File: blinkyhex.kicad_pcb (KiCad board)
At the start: 2 copper layers, 90.5 x 37.9 mm, 124 parts, among them IC1 WS2812B, IC2 ATTINY85-S, K1 D0, K2 A3, K3 A1, K4 A2, K5 reset+in, K6 D1, K7 reset, P1 act-a2, P2 act-a3, P3 act-a1, P4 act-1, P5 act-0, P6 MISO, P7 SCK, P8 MOSI, P9 ISCP

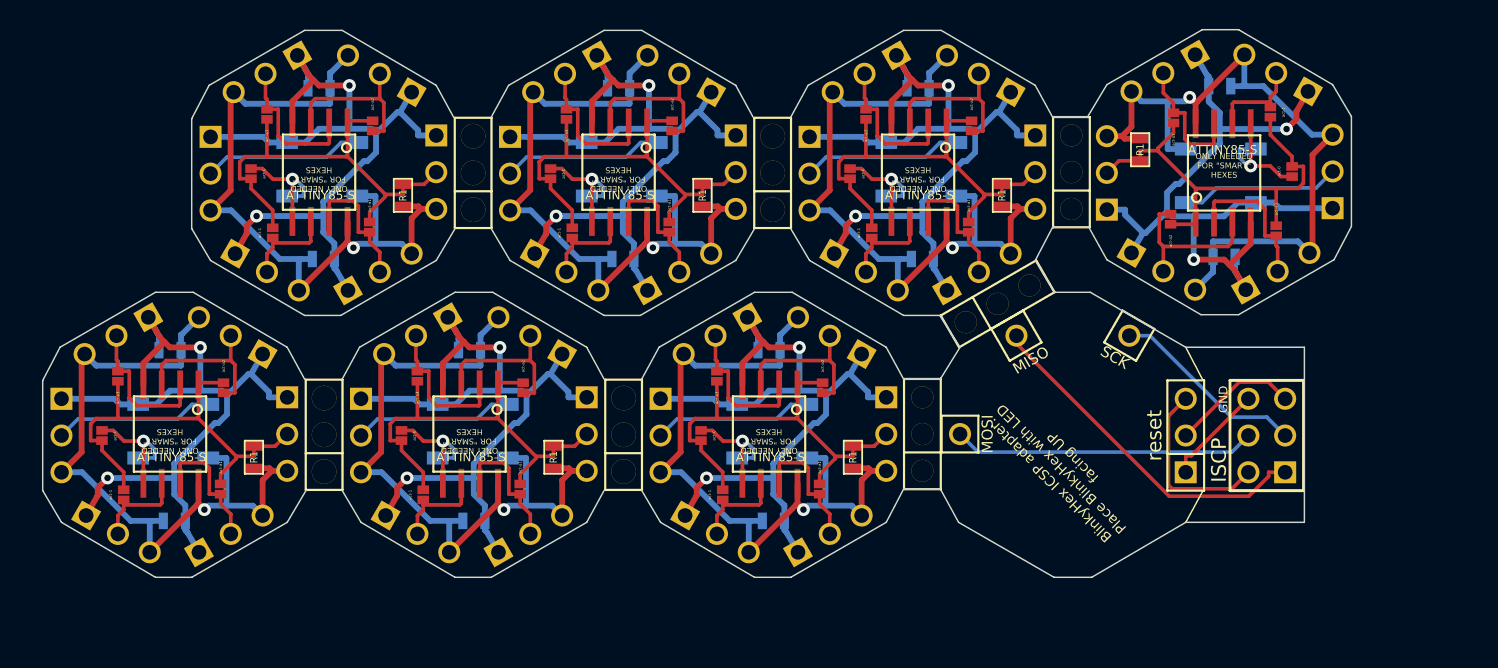
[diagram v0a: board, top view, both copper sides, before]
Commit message: Published.
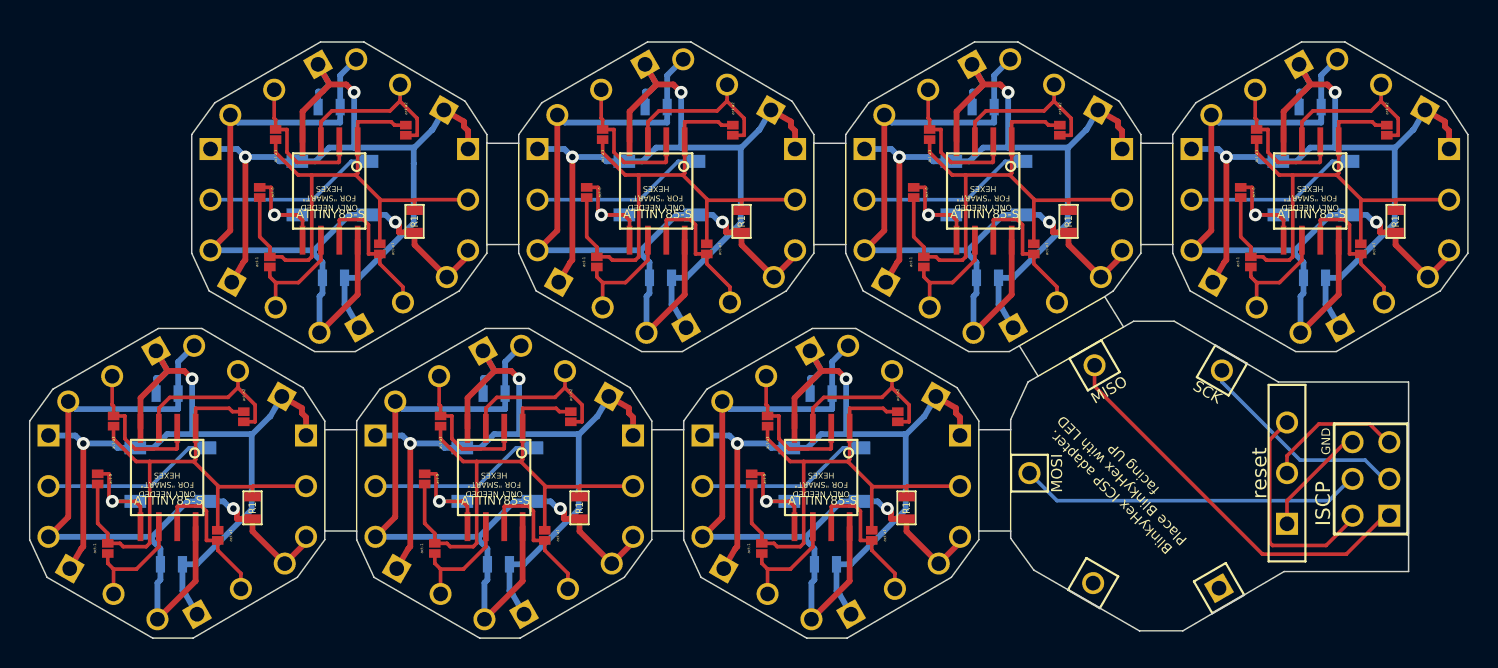
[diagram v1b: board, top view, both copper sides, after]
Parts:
- removed 2, 3, 4, PIN_ARRAY_3X1 (x4): Val**, PIN_ARRAY_3X1
- removed the C1 at (94.8, 28.6)
- removed the C1 at (22.0, 35.0)
- removed the C1 at (42.7, 35.0)
- removed the C1 at (63.4, 35.0)
- removed the C1 at (73.7, 16.9)
- removed the C1 at (53.0, 16.9)
- removed the C2 at (94.5, 16.8)
- removed the C2 at (22.3, 46.8)
- removed the C2 at (43.0, 46.8)
- removed the C2 at (63.7, 46.8)
- removed the C2 at (74.0, 28.7)
- removed the C2 at (53.3, 28.7)
- removed the IC1 at (94.7, 22.9)
- removed the IC1 at (22.2, 40.6)
- removed the IC1 at (42.9, 40.6)
- removed the IC1 at (63.6, 40.6)
- removed the IC1 at (73.9, 22.5)
- removed the IC1 at (53.2, 22.5)
- removed the IC2 at (94.8, 22.6)
- removed the IC2 at (22.1, 40.9)
- removed the IC2 at (42.8, 40.9)
- removed the IC2 at (63.5, 40.9)
- removed the IC2 at (73.8, 22.8)
- removed the IC2 at (53.1, 22.8)
- removed the K1 at (102.3, 22.6)
- removed the K1 at (14.5, 40.9)
- removed the K1 at (35.2, 40.9)
- removed the K1 at (55.9, 40.9)
- removed the K1 at (66.2, 22.8)
- removed the K1 at (45.5, 22.8)
- removed the K1 at (24.8, 22.8)
- removed the K2 at (98.5, 29.6)
- removed the K2 at (18.3, 34.0)
- removed the K2 at (39.0, 34.0)
- removed the K2 at (59.7, 34.0)
- removed the K2 at (70.0, 15.9)
- removed the K2 at (49.3, 15.9)
- removed the K2 at (28.6, 15.9)
- removed the K3 at (90.7, 15.8)
- removed the K3 at (26.2, 47.7)
- removed the K3 at (46.9, 47.7)
- removed the K3 at (67.6, 47.7)
- removed the K3 at (77.9, 29.6)
- removed the K3 at (57.2, 29.6)
- removed the K3 at (36.5, 29.6)
- removed the K4 at (90.7, 29.6)
- removed the K4 at (26.2, 34.0)
- removed the K4 at (46.9, 34.0)
- removed the K4 at (67.6, 34.0)
- removed the K4 at (77.9, 15.9)
- removed the K4 at (57.2, 15.9)
- removed the K4 at (36.5, 15.9)
- removed the K5 at (86.8, 22.8)
- removed the K5 at (30.1, 40.8)
- removed the K5 at (50.8, 40.8)
- removed the K5 at (71.5, 40.8)
- removed the K5 at (81.8, 22.7)
- removed the K5 at (61.1, 22.7)
- removed the K5 at (40.4, 22.7)
- removed the K6 at (98.5, 15.8)
- removed the K6 at (18.4, 47.7)
- removed the K6 at (39.1, 47.7)
- removed the K6 at (59.8, 47.7)
- removed the K6 at (70.1, 29.6)
- removed the K6 at (49.4, 29.6)
- removed the K6 at (28.7, 29.6)
- removed the P1 at (91.2, 25.9)
- removed the P1 at (25.7, 37.6)
- removed the P1 at (46.4, 37.6)
- removed the P1 at (67.1, 37.6)
- removed the P1 at (77.4, 19.5)
- removed the P1 at (56.7, 19.5)
- removed the P2 at (98.5, 26.8)
- removed the P2 at (18.4, 36.8)
- removed the P2 at (39.1, 36.8)
- removed the P2 at (59.8, 36.8)
- removed the P2 at (70.1, 18.7)
- removed the P2 at (49.4, 18.7)
- removed the P3 at (91.3, 18.9)
- removed the P3 at (25.5, 44.6)
- removed the P3 at (46.2, 44.6)
- removed the P3 at (66.9, 44.6)
- removed the P3 at (77.2, 26.5)
- removed the P3 at (56.5, 26.5)
- removed the P4 at (98.0, 18.6)
- removed the P4 at (18.8, 45.0)
- removed the P4 at (39.5, 45.0)
- removed the P4 at (60.2, 45.0)
- removed the P4 at (70.5, 26.9)
- removed the P4 at (49.8, 26.9)
- removed the P5 at (99.5, 22.6)
- removed the P5 at (17.3, 40.9)
- removed the P5 at (38.0, 40.9)
- removed the P5 at (58.7, 40.9)
- removed the P5 at (69.0, 22.8)
- removed the P5 at (48.3, 22.8)
- removed the R1 at (89.0, 21.1)
- removed the R1 at (27.8, 42.4)
- removed the R1 at (48.5, 42.4)
- removed the R1 at (69.2, 42.4)
- removed the R1 at (79.5, 24.3)
- removed the R1 at (58.8, 24.3)
- added 1: Val**, PIN_ARRAY_1, F.Cu at (85.8, 51.1)
- added 1: Val**, PIN_ARRAY_1, F.Cu at (94.5, 51.5)
- added C1: 0.1uf, SM0603_Capa, B.Cu at (33.0, 18.2)
- added C1: 0.1uf, SM0603_Capa, B.Cu at (55.6, 18.2)
- added C1: 0.1uf, SM0603_Capa, B.Cu at (78.2, 18.2)
- added C1: 0.1uf, SM0603_Capa, B.Cu at (67.0, 38.0)
- added C1: 0.1uf, SM0603_Capa, B.Cu at (100.8, 18.2)
- added C1: 0.1uf, SM0603_Capa, B.Cu at (44.4, 38.0)
- added C2: 1uf, SM0603_Capa, B.Cu at (33.3, 30.0)
- added C2: 1uf, SM0603_Capa, B.Cu at (55.9, 30.0)
- added C2: 1uf, SM0603_Capa, B.Cu at (78.5, 30.0)
- added C2: 1uf, SM0603_Capa, B.Cu at (67.3, 49.8)
- added C2: 1uf, SM0603_Capa, B.Cu at (101.1, 30.0)
- added C2: 1uf, SM0603_Capa, B.Cu at (44.7, 49.8)
- added IC1: WS2812B, ws2812b, B.Cu at (33.2, 23.8)
- added IC1: WS2812B, ws2812b, B.Cu at (55.8, 23.8)
- added IC1: WS2812B, ws2812b, B.Cu at (78.4, 23.8)
- added IC1: WS2812B, ws2812b, B.Cu at (67.2, 43.6)
- added IC1: WS2812B, ws2812b, B.Cu at (101.0, 23.8)
- added IC1: WS2812B, ws2812b, B.Cu at (44.6, 43.6)
- added IC2: ATTINY85-S, SOIC8_W, F.Cu at (33.1, 24.1)
- added IC2: ATTINY85-S, SOIC8_W, F.Cu at (55.7, 24.1)
- added IC2: ATTINY85-S, SOIC8_W, F.Cu at (78.3, 24.1)
- added IC2: ATTINY85-S, SOIC8_W, F.Cu at (67.1, 43.9)
- added IC2: ATTINY85-S, SOIC8_W, F.Cu at (100.9, 24.1)
- added IC2: ATTINY85-S, SOIC8_W, F.Cu at (44.5, 43.9)
- added K1: D0, pixelstrip-array, B.Cu at (24.8, 24.6)
- added K1: D0, pixelstrip-array, B.Cu at (47.4, 24.6)
- added K1: D0, pixelstrip-array, B.Cu at (70.0, 24.6)
- added K1: D0, pixelstrip-array, B.Cu at (58.8, 44.4)
- added K1: D0, pixelstrip-array, B.Cu at (92.6, 24.6)
- added K1: D0, pixelstrip-array, B.Cu at (36.2, 44.4)
- added K1: D0, pixelstrip-array, B.Cu at (13.6, 44.4)
- added K2: A3, pixelstrip-array, B.Cu at (29.2, 17.0)
- added K2: A3, pixelstrip-array, B.Cu at (51.8, 17.0)
- added K2: A3, pixelstrip-array, B.Cu at (74.4, 17.0)
- added K2: A3, pixelstrip-array, B.Cu at (63.2, 36.8)
- added K2: A3, pixelstrip-array, B.Cu at (97.0, 17.0)
- added K2: A3, pixelstrip-array, B.Cu at (40.6, 36.8)
- added K2: A3, pixelstrip-array, B.Cu at (18.0, 36.8)
- added K3: A1, pixelstrip-array, B.Cu at (38.1, 31.7)
- added K3: A1, pixelstrip-array, B.Cu at (60.7, 31.7)
- added K3: A1, pixelstrip-array, B.Cu at (83.3, 31.7)
- added K3: A1, pixelstrip-array, B.Cu at (72.1, 51.5)
- added K3: A1, pixelstrip-array, B.Cu at (105.9, 31.7)
- added K3: A1, pixelstrip-array, B.Cu at (49.5, 51.5)
- added K3: A1, pixelstrip-array, B.Cu at (26.9, 51.5)
- added K4: A2, pixelstrip-array, B.Cu at (37.9, 16.6)
- added K4: A2, pixelstrip-array, B.Cu at (60.5, 16.6)
- added K4: A2, pixelstrip-array, B.Cu at (83.1, 16.6)
- added K4: A2, pixelstrip-array, B.Cu at (71.9, 36.5)
- added K4: A2, pixelstrip-array, B.Cu at (105.7, 16.6)
- added K4: A2, pixelstrip-array, B.Cu at (49.3, 36.5)
- added K4: A2, pixelstrip-array, B.Cu at (26.7, 36.5)
- added K5: reset+in, pixelstrip-array, B.Cu at (42.6, 24.6)
- added K5: reset+in, pixelstrip-array, B.Cu at (65.2, 24.6)
- added K5: reset+in, pixelstrip-array, B.Cu at (87.8, 24.6)
- added K5: reset+in, pixelstrip-array, B.Cu at (76.6, 44.4)
- added K5: reset+in, pixelstrip-array, B.Cu at (110.4, 24.6)
- added K5: reset+in, pixelstrip-array, B.Cu at (54.0, 44.4)
- added K5: reset+in, pixelstrip-array, B.Cu at (31.4, 44.4)
- added K6: D1, pixelstrip-array, B.Cu at (29.3, 32.0)
- added K6: D1, pixelstrip-array, B.Cu at (51.9, 32.0)
- added K6: D1, pixelstrip-array, B.Cu at (74.5, 32.0)
- added K6: D1, pixelstrip-array, B.Cu at (63.3, 51.9)
- added K6: D1, pixelstrip-array, B.Cu at (97.1, 32.0)
- added K6: D1, pixelstrip-array, B.Cu at (40.7, 51.9)
- added K6: D1, pixelstrip-array, B.Cu at (18.1, 51.9)
- added P1: act-a2, 603_bridge, F.Cu at (38.3, 19.8)
- added P1: act-a2, 603_bridge, F.Cu at (60.9, 19.8)
- added P1: act-a2, 603_bridge, F.Cu at (83.5, 19.8)
- added P1: act-a2, 603_bridge, F.Cu at (72.3, 39.6)
- added P1: act-a2, 603_bridge, F.Cu at (106.1, 19.8)
- added P1: act-a2, 603_bridge, F.Cu at (49.7, 39.6)
- added P2: act-a3, 603_bridge, F.Cu at (29.3, 20.1)
- added P2: act-a3, 603_bridge, F.Cu at (51.9, 20.1)
- added P2: act-a3, 603_bridge, F.Cu at (74.5, 20.1)
- added P2: act-a3, 603_bridge, F.Cu at (63.3, 39.9)
- added P2: act-a3, 603_bridge, F.Cu at (97.1, 20.1)
- added P2: act-a3, 603_bridge, F.Cu at (40.7, 39.9)
- added P3: act-a1, 603_bridge, F.Cu at (36.5, 28.0)
- added P3: act-a1, 603_bridge, F.Cu at (59.1, 28.0)
- added P3: act-a1, 603_bridge, F.Cu at (81.7, 28.0)
- added P3: act-a1, 603_bridge, F.Cu at (70.5, 47.8)
- added P3: act-a1, 603_bridge, F.Cu at (104.3, 28.0)
- added P3: act-a1, 603_bridge, F.Cu at (47.9, 47.8)
- added P4: act-1, 603_bridge, F.Cu at (28.9, 28.9)
- added P4: act-1, 603_bridge, F.Cu at (51.5, 28.9)
- added P4: act-1, 603_bridge, F.Cu at (74.1, 28.9)
- added P4: act-1, 603_bridge, F.Cu at (62.9, 48.7)
- added P4: act-1, 603_bridge, F.Cu at (96.7, 28.9)
- added P4: act-1, 603_bridge, F.Cu at (40.3, 48.7)
- added P5: act-0, 603_bridge, F.Cu at (28.2, 24.1)
- added P5: act-0, 603_bridge, F.Cu at (50.8, 24.1)
- added P5: act-0, 603_bridge, F.Cu at (73.4, 24.1)
- added P5: act-0, 603_bridge, F.Cu at (62.2, 43.9)
- added P5: act-0, 603_bridge, F.Cu at (96.0, 24.1)
- added P5: act-0, 603_bridge, F.Cu at (39.6, 43.9)
- added R1: 10k, SM0603, F.Cu at (38.9, 26.1)
- added R1: 10k, SM0603, F.Cu at (61.5, 26.1)
- added R1: 10k, SM0603, F.Cu at (84.1, 26.1)
- added R1: 10k, SM0603, F.Cu at (72.9, 45.9)
- added R1: 10k, SM0603, F.Cu at (106.7, 26.1)
- added R1: 10k, SM0603, F.Cu at (50.3, 45.9)
- K7: footprint PIN_ARRAY_3X1 -> pixelstrip-array
- moved P4 24.6 mm to (17.7, 48.7)
- moved R1 24.0 mm to (27.7, 45.9)
- moved P3 23.7 mm to (25.3, 47.8)
- moved P2 23.7 mm to (18.1, 39.9)
- moved P5 23.6 mm to (17.0, 43.9)
- moved C1 23.6 mm to (21.8, 38.0)
- moved IC1 23.6 mm to (22.0, 43.6)
- moved C2 23.6 mm to (22.1, 49.8)
- moved IC2 23.6 mm to (21.9, 43.9)
- moved P1 22.0 mm to (27.1, 39.6)
- moved P9 7.80 mm to (105.0, 43.9)
- moved K7 7.47 mm to (99.2, 43.5)
- moved P7 6.84 mm to (94.7, 36.4)
- moved P6 5.78 mm to (85.9, 36.0)
- moved P8 5.51 mm to (81.4, 43.5)
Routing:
- net reset: track 216.2 -> 277.3 mm
- net GND: track 377.5 -> 432.4 mm
- net +5V: track 362.7 -> 409.1 mm
- net 1: track 46.0 -> 56.8 mm
- net A1: track 64.4 -> 72.7 mm
- net A2: track 77.9 -> 85.5 mm
- net 0: track 61.8 -> 54.9 mm
- net 0+1: track 77.3 -> 83.6 mm
- net N-000007: track 24.3 -> 27.7 mm
- net N-000009: track 12.6 -> 15.6 mm
- net N-0000012: track 20.9 -> 23.7 mm
- net N-0000011: track 13.6 -> 15.1 mm
- net A3: track 71.9 -> 73.2 mm
- net N-0000010: track 8.88 -> 9.70 mm
- net N-000008: track 7.10 -> 7.80 mm
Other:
- board size 90.5 x 37.9 mm -> 99.4 x 41.2 mm
